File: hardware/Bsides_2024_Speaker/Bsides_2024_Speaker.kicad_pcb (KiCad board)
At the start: 2 copper layers, 144.4 x 144.3 mm, 63 parts, among them J1 Add_On, J2 Battery, J3 Battery, J4 OLED, J5 Serial_IN, J6 Serial_OUT, P1 USB_C_Plug_USB2.0, Q1 DMG3415U-7, SW1 ON, SW2 SW, SW3 BOOT, SW4 SW, SW5 SW, SW6 SW, SW7 SW, U1 ESP32-C6-WROOM-1-N4, U2 AP2112K-3.3

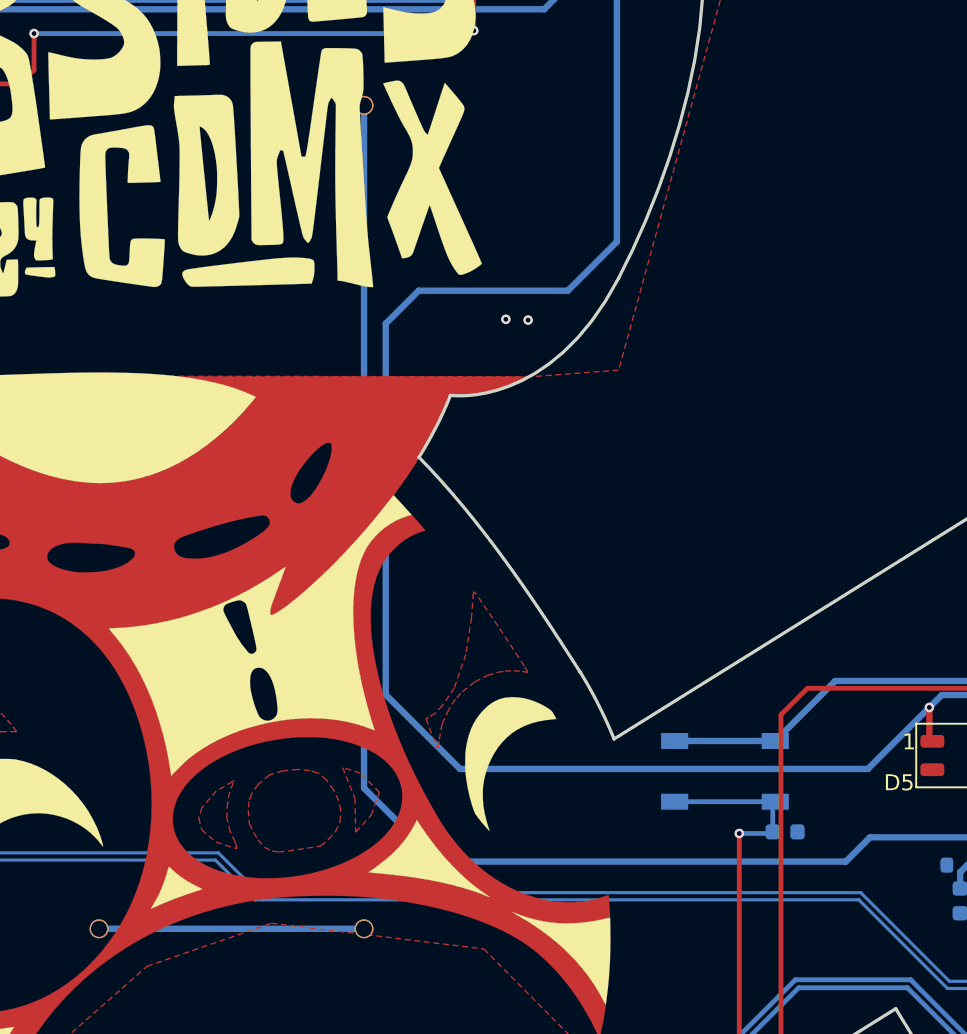
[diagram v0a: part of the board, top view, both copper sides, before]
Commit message: feat(Hw): Labels added
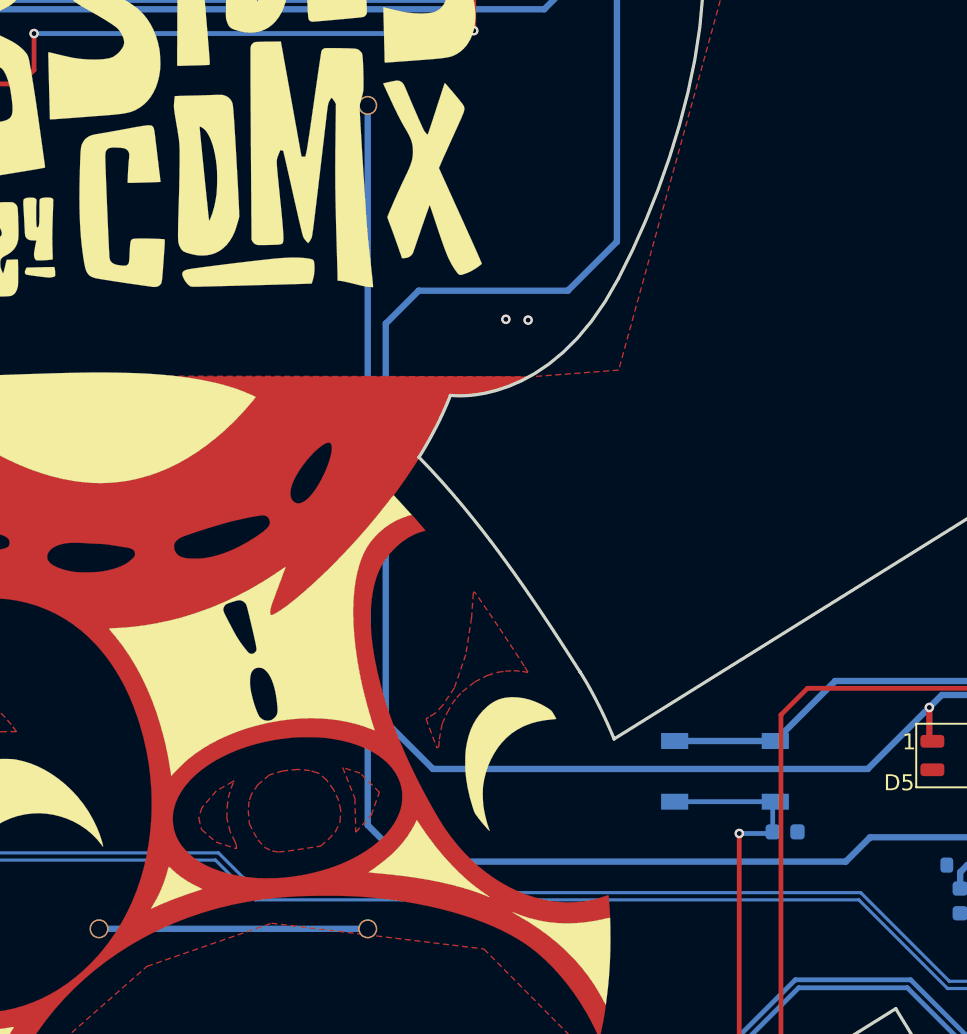
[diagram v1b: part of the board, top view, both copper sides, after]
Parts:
- moved J2 0.23 mm to (154.1, 76.9)
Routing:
- net +BATT: track 89.6 -> 91.0 mm
- net /VOUT: track 432.9 -> 433.9 mm
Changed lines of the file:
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@@
 	(footprint "bsides:BH-AA-A1AJ020"
 		(layer "B.Cu")
-		(at 153.88 76.875 -90)
+		(at 154.11 76.875 -90)
 		(property "Reference" "J2"
 			(at 0 0.5 90)
@@
 	)
 	(segment
-		(start 162.93 34.88)
-		(end 166.41 34.88)
-		(width 0.4)
-		(layer "B.Cu")
-		(net 3)
-	)
-	(segment
 		(start 111.52 98.485)
 		(end 111.4 98.605)
@@
 	)
 	(segment
-		(start 166.64 62.7)
-		(end 157.3 62.7)
+		(start 162.93 34.88)
+		(end 166.41 34.88)
 		(width 0.4)
 		(layer "B.Cu")
@@
 	)
 	(segment
+		(start 169.71 38.18)
+		(end 169.71 59.63)
+		(width 0.4)
+		(layer "B.Cu")
+		(net 3)
+	)
+	(segment
 		(start 118.38 72.39)
 		(end 118.38 72.49)
@@
 	)
 	(segment
-		(start 162.59 35.22)
-		(end 162.93 34.88)
-		(width 0.4)
-		(layer "B.Cu")
-		(net 3)
-	)
-	(segment
 		(start 160.55 42.9)
 		(end 158.97 44.48)
@@
 	)
 	(segment
-		(start 159.89 92.64)
-		(end 185.42 92.64)
+		(start 120.1775 95.9125)
+		(end 120.1775 96.8975)
 		(width 0.4)
 		(layer "B.Cu")
@@
 	)
 	(segment
-		(start 120.1775 95.9125)
-		(end 120.1775 96.8975)
+		(start 155.24 64.76)
+		(end 155.24 89.69)
 		(width 0.4)
 		(layer "B.Cu")
@@
 	)
 	(segment
-		(start 169.71 59.63)
-		(end 166.64 62.7)
-		(width 0.4)
-		(layer "B.Cu")
-		(net 3)
-	)
-	(segment
 		(start 93.29 140.1)
 		(end 115.2 140.1)
@@
 	)
 	(segment
-		(start 166.41 34.88)
-		(end 169.71 38.18)
-		(width 0.4)
-		(layer "B.Cu")
-		(net 3)
-	)
-	(segment
 		(start 111.85 94.74)
 		(end 112.4 95.29)
@@
 	)
 	(segment
-		(start 169.71 38.18)
-		(end 169.71 59.63)
+		(start 162.59 35.22)
+		(end 162.93 34.88)
 		(width 0.4)
 		(layer "B.Cu")
@@
 	)
 	(segment
+		(start 162.59 38.2)
+		(end 162.59 35.22)
+		(width 0.4)
+		(layer "B.Cu")
+		(net 3)
+	)
+	(segment
 		(start 128.7 69.22)
 		(end 128.7 69.08)
@@
 	)
 	(segment
+		(start 169.71 59.63)
+		(end 166.64 62.7)
+		(width 0.4)
+		(layer "B.Cu")
+		(net 3)
+	)
+	(segment
 		(start 118.86 71.91)
 		(end 121.73 71.91)
@@
 	)
 	(segment
-		(start 185.42 92.64)
-		(end 189.27 88.79)
+		(start 155.24 89.69)
+		(end 158.19 92.64)
 		(width 0.4)
 		(layer "B.Cu")
@@
 	)
 	(segment
+		(start 185.42 92.64)
+		(end 189.27 88.79)
+		(width 0.4)
+		(layer "B.Cu")
+		(net 3)
+	)
+	(segment
 		(start 120.48 44.48)
 		(end 119.91 43.91)
@@
 	)
 	(segment
-		(start 155.24 87.99)
-		(end 159.89 92.64)
-		(width 0.4)
-		(layer "B.Cu")
-		(net 3)
-	)
-	(segment
 		(start 157.3 62.7)
 		(end 155.24 64.76)
@@
 	)
 	(segment
+		(start 158.19 92.64)
+		(end 185.42 92.64)
+		(width 0.4)
+		(layer "B.Cu")
+		(net 3)
+	)
+	(segment
 		(start 92.235 156.64)
 		(end 92.2 156.605)
@@
 	)
 	(segment
-		(start 155.24 64.76)
-		(end 155.24 87.99)
+		(start 166.64 62.7)
+		(end 157.3 62.7)
 		(width 0.4)
 		(layer "B.Cu")
@@
 	)
 	(segment
-		(start 162.59 38.2)
-		(end 162.59 35.22)
-		(width 0.4)
-		(layer "B.Cu")
-		(net 3)
-	)
-	(segment
 		(start 193.065 88.01)
 		(end 193.065 92.27495)
@@
 	)
 	(segment
+		(start 166.41 34.88)
+		(end 169.71 38.18)
+		(width 0.4)
+		(layer "B.Cu")
+		(net 3)
+	)
+	(segment
 		(start 129.11 50.08)
 		(end 129.11 68.19)
@@
 	)
 	(segment
-		(start 184.04 98.44)
-		(end 185.56 96.92)
+		(start 154.11 51.1)
+		(end 154.11 96.16)
 		(width 0.4)
 		(layer "B.Cu")
@@
 	)
 	(segment
-		(start 153.88 93.84)
-		(end 158.48 98.44)
+		(start 154.11 96.16)
+		(end 156.39 98.44)
 		(width 0.4)
 		(layer "B.Cu")
@@
 	)
 	(segment
-		(start 153.891847 51.111847)
-		(end 153.88 51.1)
+		(start 153.903694 51.1)
+		(end 154.11 51.1)
+		(width 0.4)
+		(layer "B.Cu")
+		(net 20)
+	)
+	(segment
+		(start 185.56 96.92)
+		(end 198.235 96.92)
 		(width 0.4)
 		(layer "B.Cu")
@@
 	)
 	(segment
-		(start 158.48 98.44)
+		(start 156.39 98.44)
 		(end 184.04 98.44)
 		(width 0.4)
@@
 	)
 	(segment
-		(start 153.88 51.1)
-		(end 153.88 93.84)
+		(start 184.04 98.44)
+		(end 185.56 96.92)
 		(width 0.4)
 		(layer "B.Cu")
@@
 	)
 	(segment
-		(start 185.56 96.92)
-		(end 198.235 96.92)
+		(start 153.891847 51.111847)
+		(end 153.903694 51.1)
 		(width 0.4)
 		(layer "B.Cu")
@@
 	)
 	(segment
-		(start 153.879107 102.649107)
-		(end 153.88 102.65)
-		(width 0.2)
+		(start 154.109107 102.649107)
+		(end 154.11 102.65)
+		(width 0.4)
 		(layer "B.Cu")
 		(net 21)
@@
 	(segment
 		(start 137.288153 102.649107)
-		(end 153.879107 102.649107)
+		(end 154.109107 102.649107)
 		(width 0.4)
 		(layer "B.Cu")
